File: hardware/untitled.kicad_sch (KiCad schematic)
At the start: 29 parts, among them U3 MC7812BDTRKG, U4 AZ1117CD-3.3TRG1, U5 AZ1117CD-3.3TRG1

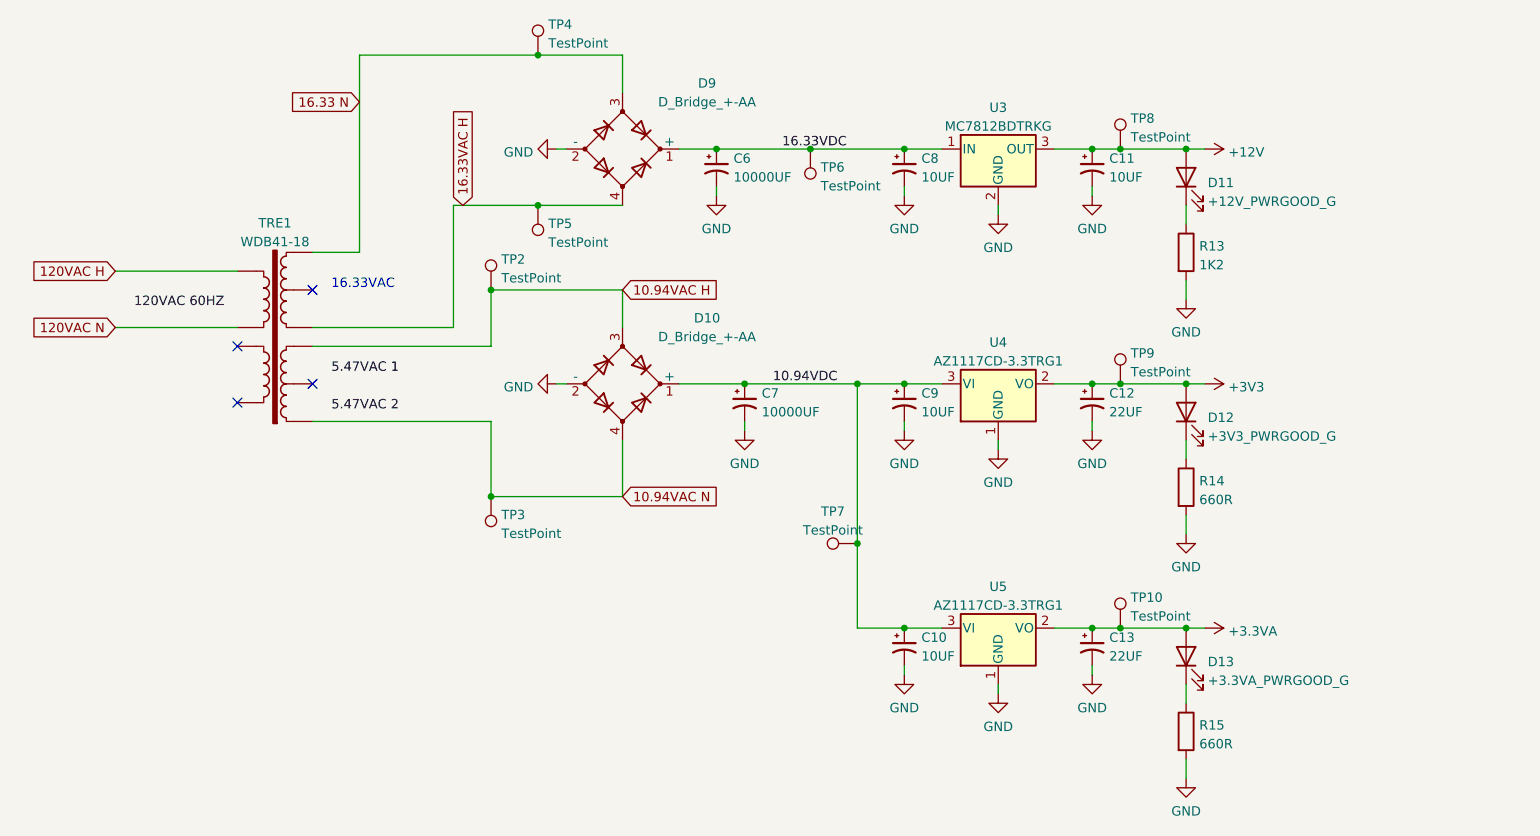
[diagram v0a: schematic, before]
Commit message: minor hardware refactoring
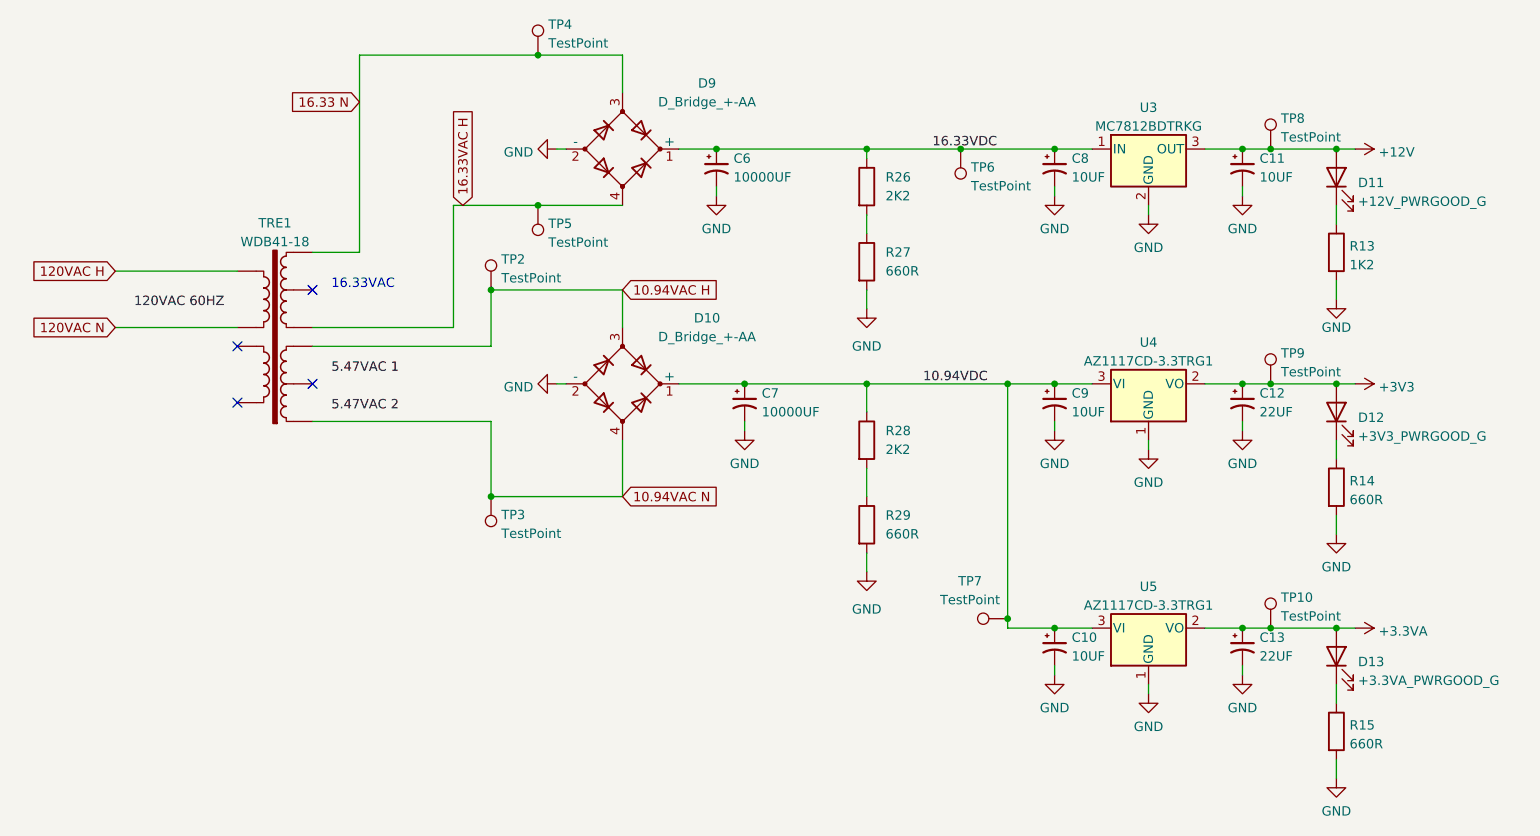
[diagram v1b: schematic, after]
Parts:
- added R26, R28: 2K2, Resistor_SMD:R_0603_1608Metric, symbol Device:R
- added R27, R29: 660R, Resistor_SMD:R_0603_1608Metric, symbol Device:R
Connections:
- net 10.94VDC: now also R28.1
- net 16.33VDC: now also R26.1
- net GND: now also R27.2, R29.2
- new net: R28.2, R29.1
- new net: R26.2, R27.1
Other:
- moved on the sheet: C10, C11, C12, C13, C8, C9, D11, D12, D13, R13, R14, R15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
